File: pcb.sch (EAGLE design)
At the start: 13 parts, among them J1 455-1750-1-ND, J2 AUDIO_JACK_TRRSSMD_RA, U1 ESP-WROVER-32ESP-WROVER-32, X1 MAB5SH

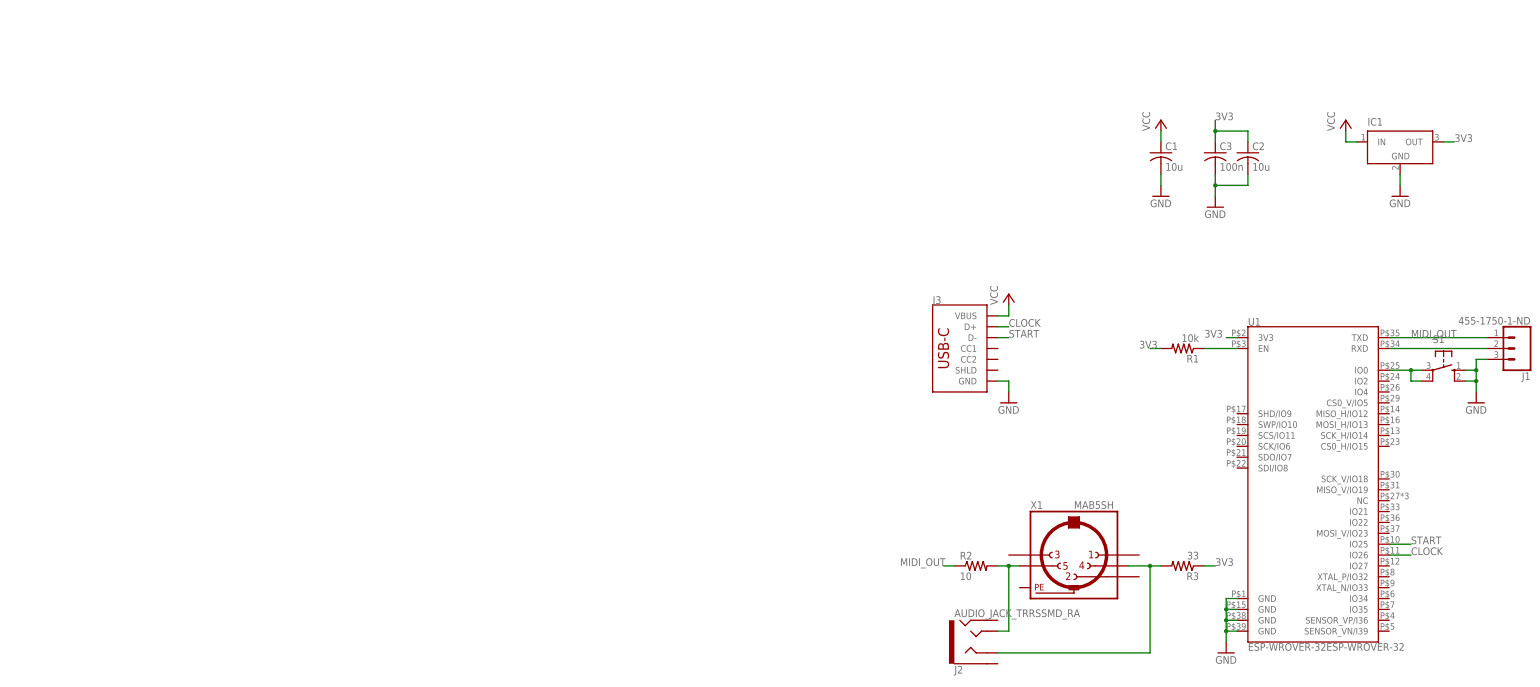
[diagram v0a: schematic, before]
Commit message: small fixes
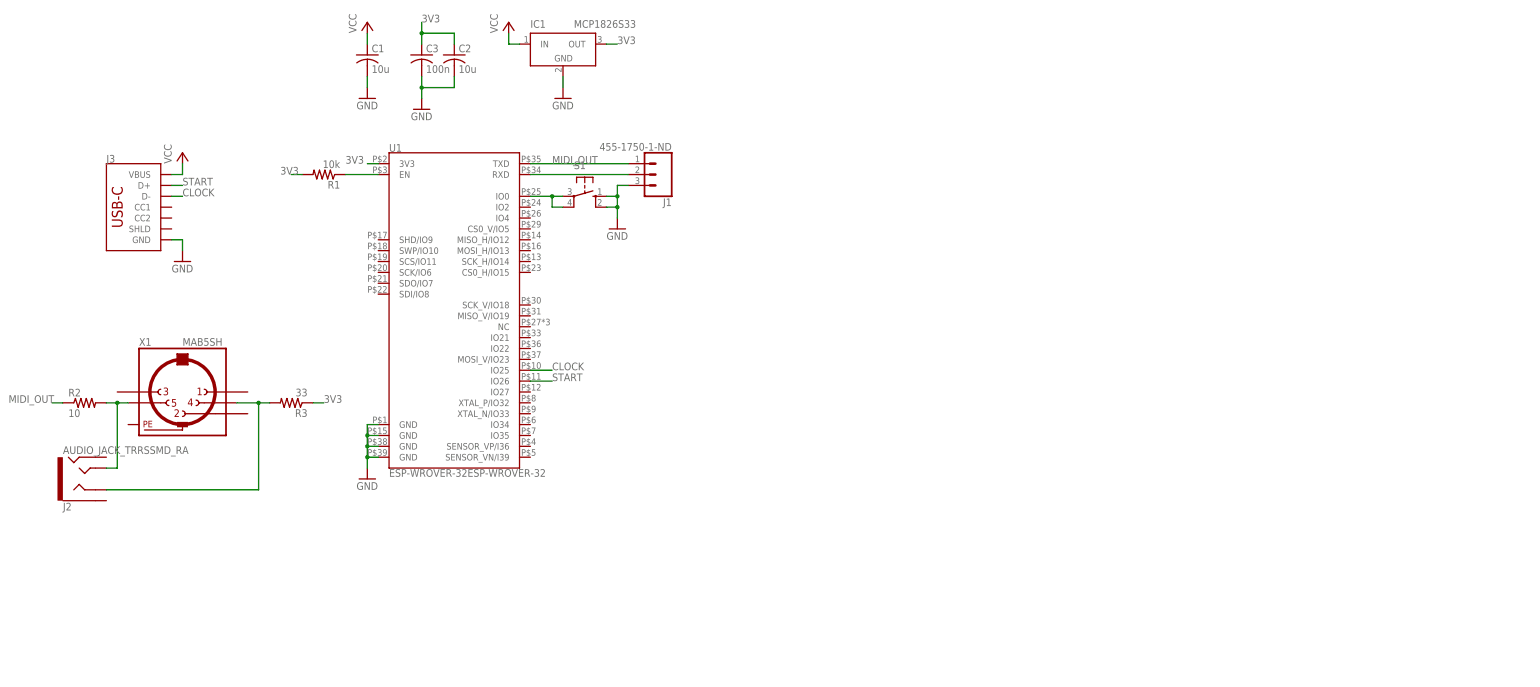
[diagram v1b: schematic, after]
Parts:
- IC1: value (none) -> MCP1826S33
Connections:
- net CLOCK: now also J3.D-, U1.IO25; no longer J3.D+, U1.IO26
- net START: now also J3.D+, U1.IO26; no longer J3.D-, U1.IO25
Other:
- moved on the sheet: C1, C2, C3, IC1, J1, J2, J3, R1, R2, R3, S1, U1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
